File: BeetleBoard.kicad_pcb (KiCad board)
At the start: 2 copper layers, 129 x 71.5 mm, 61 parts, among them J1 Battery Connector, J10 VBAT_ESC_C, J11 VBAT_ESC_E, J12 VBAT_ESC_F, J13 VBAT_ESC_G, J14 VBAT_ESC_D, J15 VBAT_ESC_H, J16 ESC G, J17 ESC H, J18 ELRS Reciever, J2 ESC A, J3 ESC B, J4 ESC C, J5 ESC D, J6 ESC E, J7 ESC F, J8 VBAT_ESC_A, J9 VBAT_ESC_B, SW1 FingerTech Switch, U1 XIAO-ESP32-C6-SMD, U2 TPS563200, U3 LSM6DSV320XTR

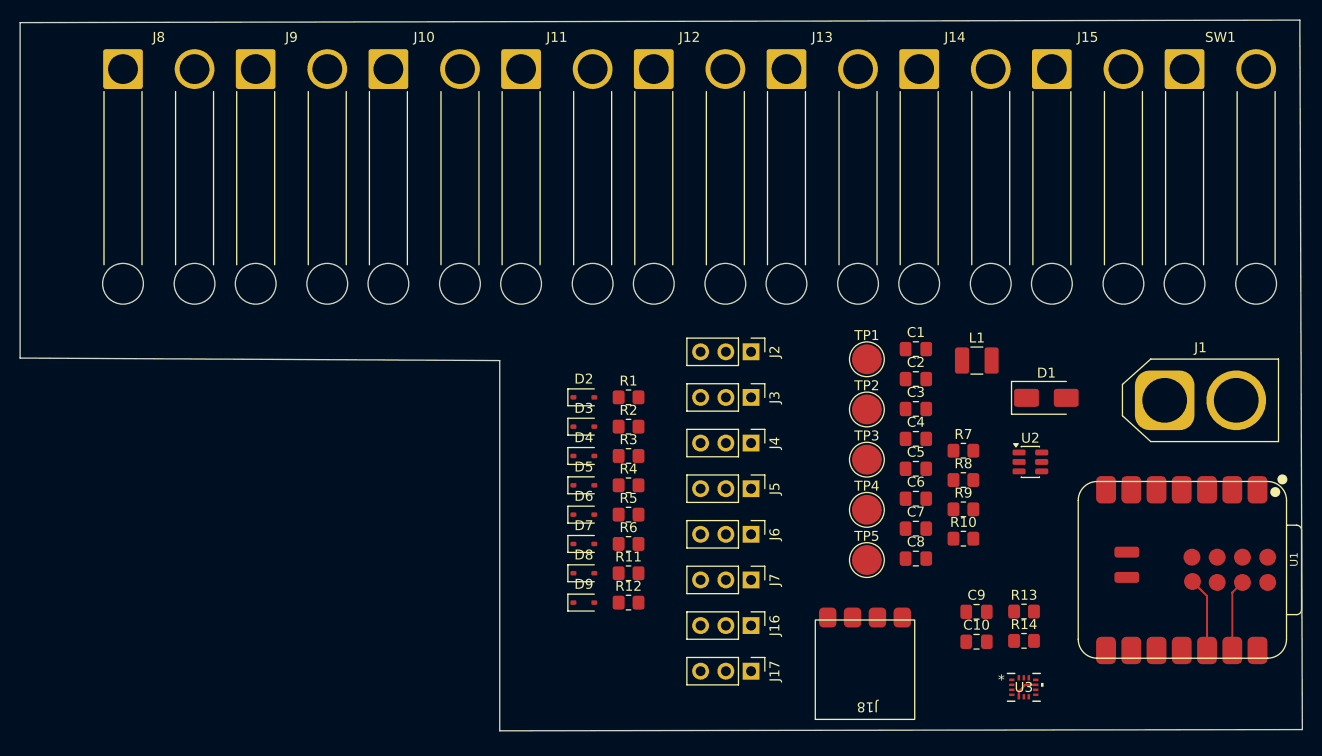
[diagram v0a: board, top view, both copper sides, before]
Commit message: redo layout and wire it up
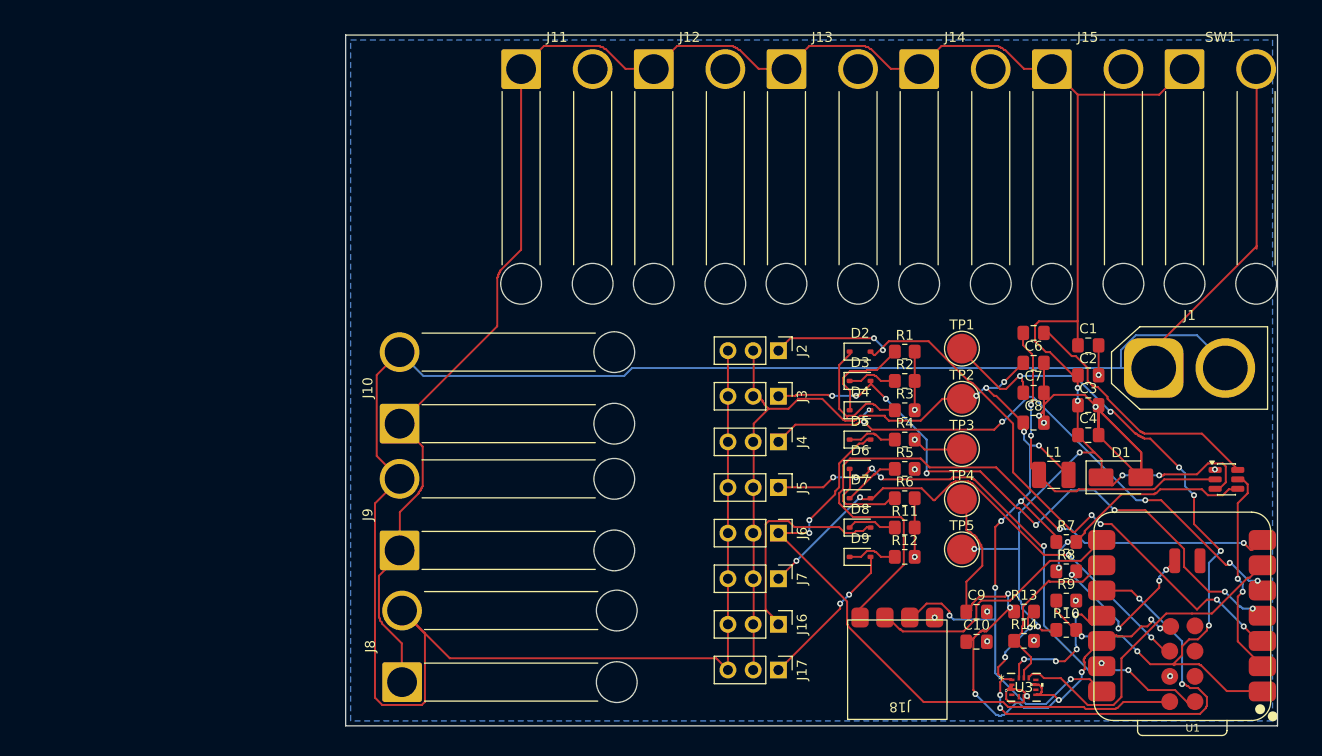
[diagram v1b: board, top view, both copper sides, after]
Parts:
- moved J8 67.8 mm to (138.4, 137.6), turned to 90 degrees
- moved J9 50.5 mm to (138.2, 124.3), turned to 90 degrees
- moved J10 35.7 mm to (138.2, 111.6), turned to 90 degrees
- moved D2 28.2 mm to (184.5, 104.3)
- moved D3 28.2 mm to (184.5, 107.3)
- moved D4 28.2 mm to (184.5, 110.2)
- moved D5 28.2 mm to (184.5, 113.2)
- moved D6 28.2 mm to (184.5, 116.2)
- moved D7 28.2 mm to (184.5, 119.1)
- moved D8 28.2 mm to (184.5, 122.0)
- moved D9 28.2 mm to (184.5, 125.0)
- moved R1 28.2 mm to (189.0, 104.3)
- moved R11 28.2 mm to (189.0, 122.0)
- moved R12 28.2 mm to (189.0, 125.0)
- moved R2 28.2 mm to (189.0, 107.3)
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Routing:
- net GND: track 7.27 -> 299.8 mm, vias 0 -> 22
- net VBUS: track 0.00 -> 242.3 mm, vias 0 -> 7
- net +5V: track 0.00 -> 130.6 mm, vias 0 -> 10
- net /VBAT_SNS: track 0.00 -> 79.2 mm, vias 0 -> 8
- net /ESC_A: track 0.00 -> 69.6 mm, vias 0 -> 6
- net /XIAO_TX: track 0.00 -> 68.1 mm, vias 0 -> 2
- net /ESC_B: track 0.00 -> 65.1 mm, vias 0 -> 8
- net /ESC_E: track 0.00 -> 64.1 mm, vias 0 -> 2
- net /ESC_C: track 0.00 -> 61.3 mm, vias 0 -> 6
- net /ESC_D: track 0.00 -> 57.2 mm, vias 0 -> 6
- net +3V3: track 10.1 -> 64.8 mm, vias 0 -> 8
- net /SPI_MISO: track 0.00 -> 52.0 mm, vias 0 -> 6
- net /ESC_F: track 0.00 -> 51.9 mm, vias 0 -> 4
- net Net-(J1-Pin_1): track 0.00 -> 34.5 mm
- net /Power/SW: track 0.00 -> 34.0 mm, vias 0 -> 2
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- added copper zone on B.Cu, net GND
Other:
- board size 129 x 71.5 mm -> 93.8 x 69.5 mm
